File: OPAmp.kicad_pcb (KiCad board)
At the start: 2 copper layers, 100 x 100 mm, 20 parts, among them Q1 TIP120, Q2 TIP125, Q3 2N2219, Q4 2N2219

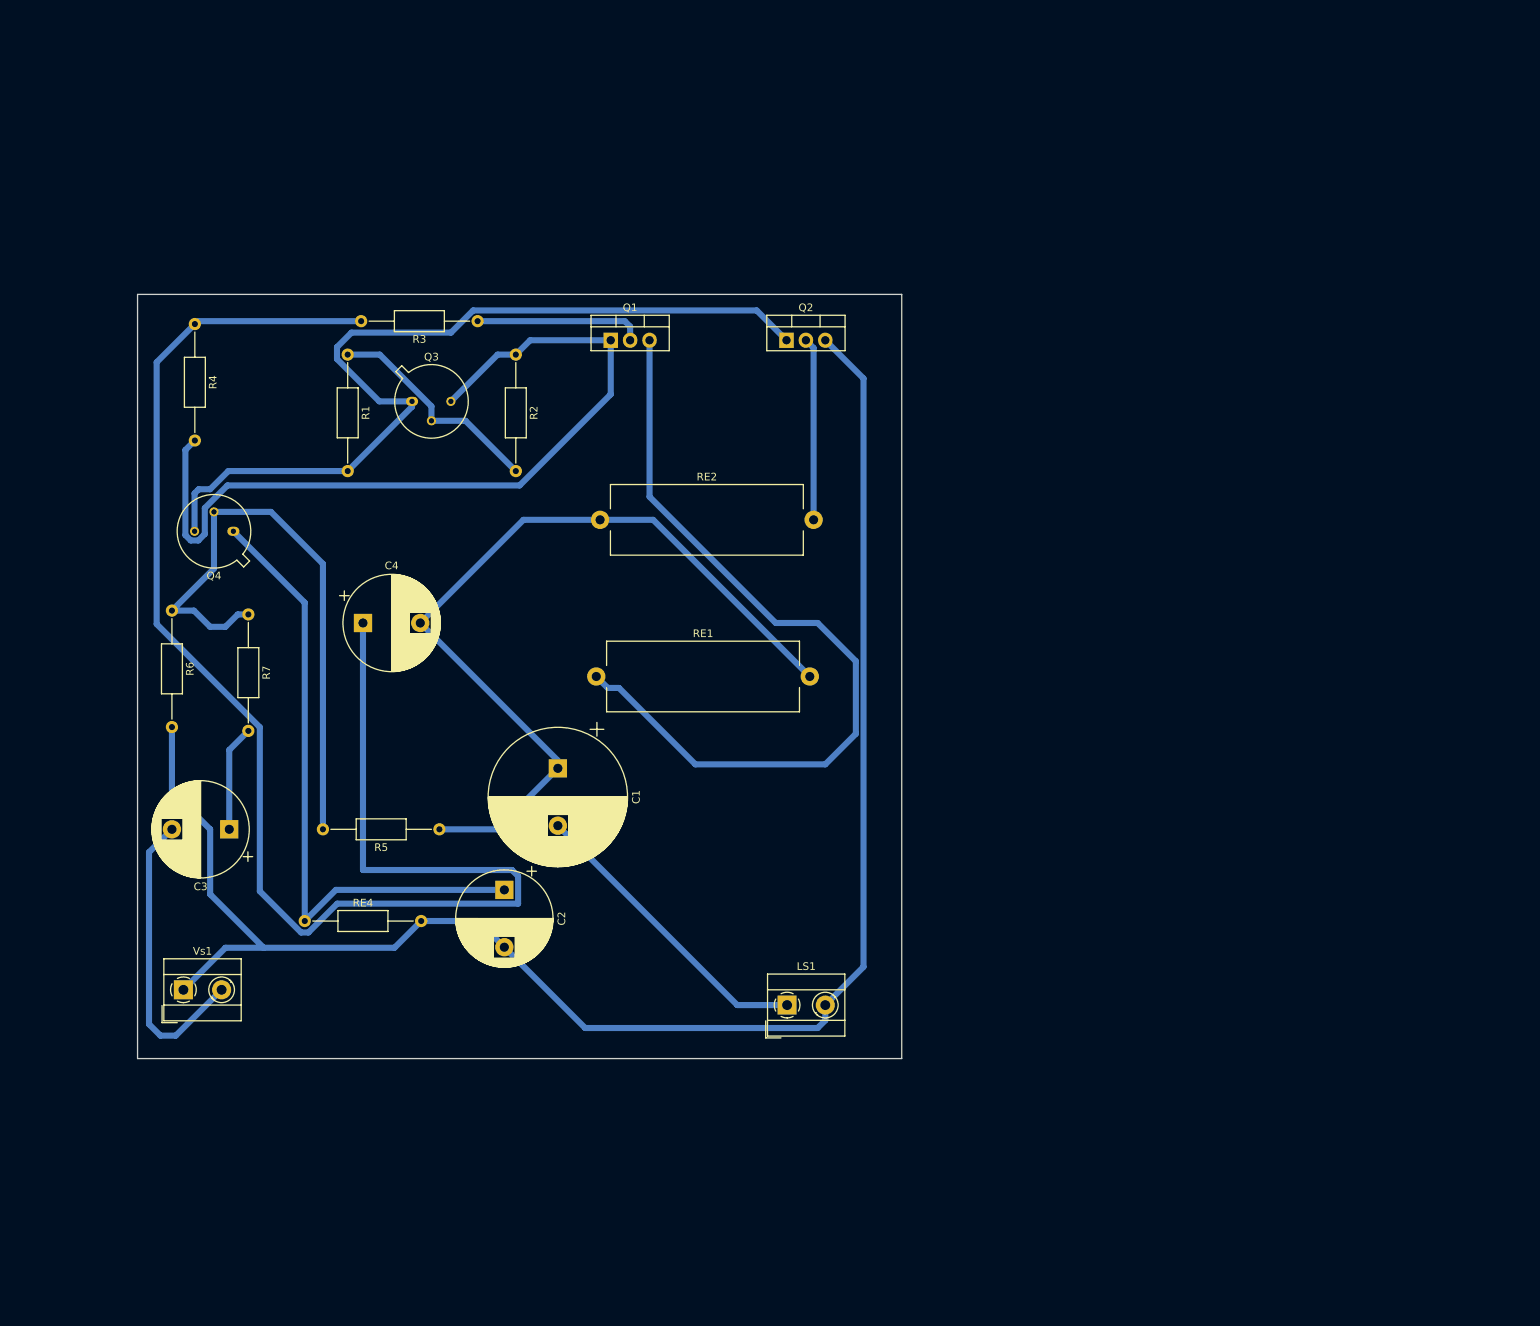
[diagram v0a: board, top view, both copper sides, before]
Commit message: Version 2
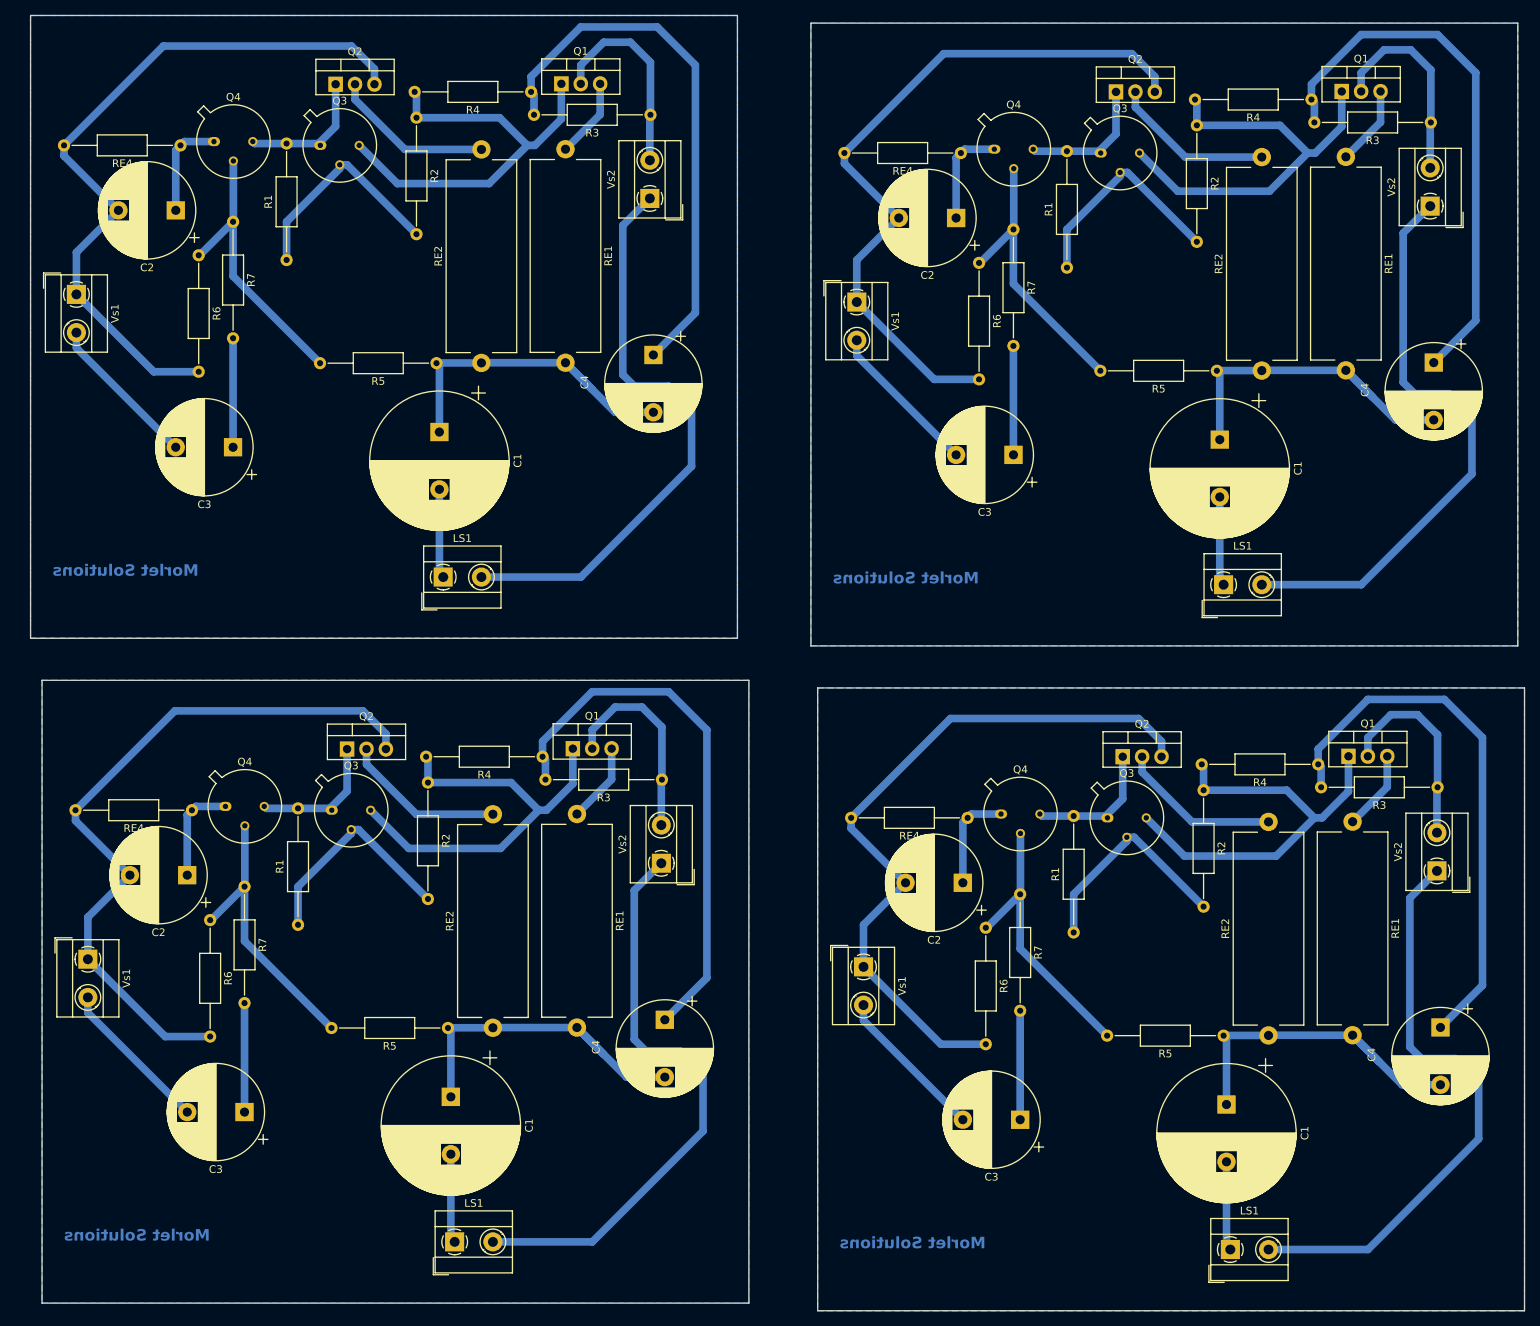
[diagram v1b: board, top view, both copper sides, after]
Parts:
- added C1: 4700uF, Capacitor_THT:CP_Radial_D18.0mm_P7.50mm, F.Cu at (142.0, 155.0)
- added C1: 4700uF, Capacitor_THT:CP_Radial_D18.0mm_P7.50mm, F.Cu at (140.5, 68.0)
- added C1: 4700uF, Capacitor_THT:CP_Radial_D18.0mm_P7.50mm, F.Cu at (243.5, 156.0)
- added C2: 100uF, Capacitor_THT:CP_Radial_D12.5mm_P7.50mm, F.Cu at (209.0, 127.0)
- added C2: 100uF, Capacitor_THT:CP_Radial_D12.5mm_P7.50mm, F.Cu at (106.0, 39.0)
- added C2: 100uF, Capacitor_THT:CP_Radial_D12.5mm_P7.50mm, F.Cu at (107.5, 126.0)
- added C3: 100uF, Capacitor_THT:CP_Radial_D12.5mm_P7.50mm, F.Cu at (115.0, 157.0)
- added C3: 100uF, Capacitor_THT:CP_Radial_D12.5mm_P7.50mm, F.Cu at (216.5, 158.0)
- added C3: 100uF, Capacitor_THT:CP_Radial_D12.5mm_P7.50mm, F.Cu at (113.5, 70.0)
- added C4: 100uF, Capacitor_THT:CP_Radial_D12.5mm_P7.50mm, F.Cu at (170.0, 144.9)
- added C4: 100uF, Capacitor_THT:CP_Radial_D12.5mm_P7.50mm, F.Cu at (168.5, 57.9)
- added C4: 100uF, Capacitor_THT:CP_Radial_D12.5mm_P7.50mm, F.Cu at (271.5, 145.9)
- added LS1: 8Ohm, TerminalBlock_MetzConnect:TerminalBlock_MetzConnect_Type055_RT01502HDWU_1x02_P5.00mm_Horizontal, F.Cu at (142.5, 174.0)
- added LS1: 8Ohm, TerminalBlock_MetzConnect:TerminalBlock_MetzConnect_Type055_RT01502HDWU_1x02_P5.00mm_Horizontal, F.Cu at (141.0, 87.0)
- added LS1: 8Ohm, TerminalBlock_MetzConnect:TerminalBlock_MetzConnect_Type055_RT01502HDWU_1x02_P5.00mm_Horizontal, F.Cu at (244.0, 175.0)
- added Q1: TIP120, Package_TO_SOT_THT:TO-220-3_Vertical, F.Cu at (156.5, 22.4)
- added Q1: TIP120, Package_TO_SOT_THT:TO-220-3_Vertical, F.Cu at (158.0, 109.4)
- added Q1: TIP120, Package_TO_SOT_THT:TO-220-3_Vertical, F.Cu at (259.5, 110.4)
- added Q2: TIP125, Package_TO_SOT_THT:TO-220-3_Vertical, F.Cu at (229.9, 110.5)
- added Q2: TIP125, Package_TO_SOT_THT:TO-220-3_Vertical, F.Cu at (128.4, 109.5)
- added Q2: TIP125, Package_TO_SOT_THT:TO-220-3_Vertical, F.Cu at (126.9, 22.5)
- added Q3: 2N2219, Package_TO_SOT_THT:TO-39-3, F.Cu at (124.9, 30.5)
- added Q3: 2N2219, Package_TO_SOT_THT:TO-39-3, F.Cu at (227.9, 118.5)
- added Q3: 2N2219, Package_TO_SOT_THT:TO-39-3, F.Cu at (126.4, 117.5)
- added Q4: 2N2219, Package_TO_SOT_THT:TO-39-3, F.Cu at (111.0, 30.0)
- added Q4: 2N2219, Package_TO_SOT_THT:TO-39-3, F.Cu at (112.5, 117.0)
- added Q4: 2N2219, Package_TO_SOT_THT:TO-39-3, F.Cu at (214.0, 118.0)
- added R1: 1kOhm, Resistor_THT:R_Axial_DIN0207_L6.3mm_D2.5mm_P15.24mm_Horizontal, F.Cu at (122.0, 132.5)
- added R1: 1kOhm, Resistor_THT:R_Axial_DIN0207_L6.3mm_D2.5mm_P15.24mm_Horizontal, F.Cu at (223.5, 133.5)
- added R1: 1kOhm, Resistor_THT:R_Axial_DIN0207_L6.3mm_D2.5mm_P15.24mm_Horizontal, F.Cu at (120.5, 45.5)
- added R2: 2.7kOhm, Resistor_THT:R_Axial_DIN0207_L6.3mm_D2.5mm_P15.24mm_Horizontal, F.Cu at (240.5, 114.9)
- added R2: 2.7kOhm, Resistor_THT:R_Axial_DIN0207_L6.3mm_D2.5mm_P15.24mm_Horizontal, F.Cu at (139.0, 113.9)
- added R2: 2.7kOhm, Resistor_THT:R_Axial_DIN0207_L6.3mm_D2.5mm_P15.24mm_Horizontal, F.Cu at (137.5, 26.9)
- added R3: 1.8kOhm, Resistor_THT:R_Axial_DIN0207_L6.3mm_D2.5mm_P15.24mm_Horizontal, F.Cu at (169.6, 113.5)
- added R3: 1.8kOhm, Resistor_THT:R_Axial_DIN0207_L6.3mm_D2.5mm_P15.24mm_Horizontal, F.Cu at (271.1, 114.5)
- added R3: 1.8kOhm, Resistor_THT:R_Axial_DIN0207_L6.3mm_D2.5mm_P15.24mm_Horizontal, F.Cu at (168.1, 26.5)
- added R4: 1.8kOhm, Resistor_THT:R_Axial_DIN0207_L6.3mm_D2.5mm_P15.24mm_Horizontal, F.Cu at (255.5, 111.5)
- added R4: 1.8kOhm, Resistor_THT:R_Axial_DIN0207_L6.3mm_D2.5mm_P15.24mm_Horizontal, F.Cu at (154.0, 110.5)
- added R4: 1.8kOhm, Resistor_THT:R_Axial_DIN0207_L6.3mm_D2.5mm_P15.24mm_Horizontal, F.Cu at (152.5, 23.5)
- added R5: 100kOhm, Resistor_THT:R_Axial_DIN0207_L6.3mm_D2.5mm_P15.24mm_Horizontal, F.Cu at (141.6, 146.0)
- added R5: 100kOhm, Resistor_THT:R_Axial_DIN0207_L6.3mm_D2.5mm_P15.24mm_Horizontal, F.Cu at (140.1, 59.0)
- added R5: 100kOhm, Resistor_THT:R_Axial_DIN0207_L6.3mm_D2.5mm_P15.24mm_Horizontal, F.Cu at (243.1, 147.0)
- added R6: 20kOhm, Resistor_THT:R_Axial_DIN0207_L6.3mm_D2.5mm_P15.24mm_Horizontal, F.Cu at (110.5, 131.9)
- added R6: 20kOhm, Resistor_THT:R_Axial_DIN0207_L6.3mm_D2.5mm_P15.24mm_Horizontal, F.Cu at (212.0, 132.9)
- added R6: 20kOhm, Resistor_THT:R_Axial_DIN0207_L6.3mm_D2.5mm_P15.24mm_Horizontal, F.Cu at (109.0, 44.9)
- added R7: 5.1kOhm, Resistor_THT:R_Axial_DIN0207_L6.3mm_D2.5mm_P15.24mm_Horizontal, F.Cu at (113.5, 40.5)
- added R7: 5.1kOhm, Resistor_THT:R_Axial_DIN0207_L6.3mm_D2.5mm_P15.24mm_Horizontal, F.Cu at (216.5, 128.5)
- added R7: 5.1kOhm, Resistor_THT:R_Axial_DIN0207_L6.3mm_D2.5mm_P15.24mm_Horizontal, F.Cu at (115.0, 127.5)
- added RE1: 1 Ohm, Resistor_THT:R_Axial_Power_L25.0mm_W9.0mm_P27.94mm, F.Cu at (157.0, 31.0)
- added RE1: 1 Ohm, Resistor_THT:R_Axial_Power_L25.0mm_W9.0mm_P27.94mm, F.Cu at (158.5, 118.0)
- added RE1: 1 Ohm, Resistor_THT:R_Axial_Power_L25.0mm_W9.0mm_P27.94mm, F.Cu at (260.0, 119.0)
- added RE2: 1 Ohm, Resistor_THT:R_Axial_Power_L25.0mm_W9.0mm_P27.94mm, F.Cu at (147.5, 146.0)
- added RE2: 1 Ohm, Resistor_THT:R_Axial_Power_L25.0mm_W9.0mm_P27.94mm, F.Cu at (146.0, 59.0)
- added RE2: 1 Ohm, Resistor_THT:R_Axial_Power_L25.0mm_W9.0mm_P27.94mm, F.Cu at (249.0, 147.0)
- added RE4: 470 Ohm, Resistor_THT:R_Axial_DIN0207_L6.3mm_D2.5mm_P15.24mm_Horizontal, F.Cu at (108.1, 117.5)
- added RE4: 470 Ohm, Resistor_THT:R_Axial_DIN0207_L6.3mm_D2.5mm_P15.24mm_Horizontal, F.Cu at (106.6, 30.5)
- added RE4: 470 Ohm, Resistor_THT:R_Axial_DIN0207_L6.3mm_D2.5mm_P15.24mm_Horizontal, F.Cu at (209.6, 118.5)
- added Vs1: Conn_01x02, TerminalBlock_MetzConnect:TerminalBlock_MetzConnect_Type055_RT01502HDWU_1x02_P5.00mm_Horizontal, F.Cu at (94.5, 137.0)
- added Vs1: Conn_01x02, TerminalBlock_MetzConnect:TerminalBlock_MetzConnect_Type055_RT01502HDWU_1x02_P5.00mm_Horizontal, F.Cu at (93.0, 50.0)
- added Vs1: Conn_01x02, TerminalBlock_MetzConnect:TerminalBlock_MetzConnect_Type055_RT01502HDWU_1x02_P5.00mm_Horizontal, F.Cu at (196.0, 138.0)
- added Vs2: Conn_01x02, TerminalBlock_MetzConnect:TerminalBlock_MetzConnect_Type055_RT01502HDWU_1x02_P5.00mm_Horizontal, F.Cu at (168.0, 37.4)
- added Vs2: Conn_01x02, TerminalBlock_MetzConnect:TerminalBlock_MetzConnect_Type055_RT01502HDWU_1x02_P5.00mm_Horizontal, F.Cu at (169.5, 124.4)
- added Vs2: Conn_01x02, TerminalBlock_MetzConnect:TerminalBlock_MetzConnect_Type055_RT01502HDWU_1x02_P5.00mm_Horizontal, F.Cu at (270.2, 38.4)
- added Vs2: Conn_01x02, TerminalBlock_MetzConnect:TerminalBlock_MetzConnect_Type055_RT01502HDWU_1x02_P5.00mm_Horizontal, F.Cu at (271.0, 125.4)
- moved R4 149.0 mm to (254.6, 24.5), turned to 180 degrees
- moved C4 144.2 mm to (270.6, 58.9), turned to -90 degrees
- moved RE4 132.2 mm to (208.7, 31.5), turned to 180 degrees
- moved R3 127.4 mm to (270.2, 27.5)
- moved Vs1 126.0 mm to (195.1, 51.0), turned to -90 degrees
- moved RE1 119.4 mm to (259.1, 32.0), turned to -90 degrees
- moved R5 118.1 mm to (242.2, 60.0)
- moved R6 115.0 mm to (211.1, 45.9)
- moved C3 113.7 mm to (215.6, 71.0)
- moved R7 112.1 mm to (215.6, 41.5)
- moved Q4 111.4 mm to (213.1, 31.0), turned to 0 degrees
- moved C2 106.0 mm to (208.1, 40.0), turned to 180 degrees
- moved Q1 101.0 mm to (258.6, 23.4)
- moved C1 96.7 mm to (242.6, 69.0)
- moved Q3 95.8 mm to (227.0, 31.5)
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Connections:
- net VCC renamed Net-(Q1-C)
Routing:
- net GND: track 220.9 -> 682.2 mm
- net Net-(Q1-B): track 110.1 -> 224.4 mm
- net Net-(C4-Pad1): track 198.0 -> 286.5 mm
- net Net-(Q3-B): track 29.4 -> 116.6 mm
- net Net-(Q1-C): track 22.0 -> 107.5 mm
- net Net-(Q4-B): track 78.6 -> 150.0 mm
- net Net-(C1-Pad1): track 110.3 -> 180.8 mm
- net Net-(Q1-E): track 106.3 -> 41.7 mm
- net Net-(Q2-C): track 23.9 -> 85.0 mm
- net Net-(Q2-B): track 114.9 -> 70.9 mm
- net Net-(C3-Pad1): track 13.9 -> 57.0 mm
- net Net-(Vs1-Pin_2): track 39.3 -> 81.5 mm
- net Net-(Q4-E): track 82.7 -> 53.4 mm
- net Net-(C1-Pad2): track 39.7 -> 46.7 mm
- added copper zone on B.Cu, net GND
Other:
- board size 100 x 100 mm -> 195.5 x 169.5 mm
- board text added: "Morlet Solutions"

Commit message: V3
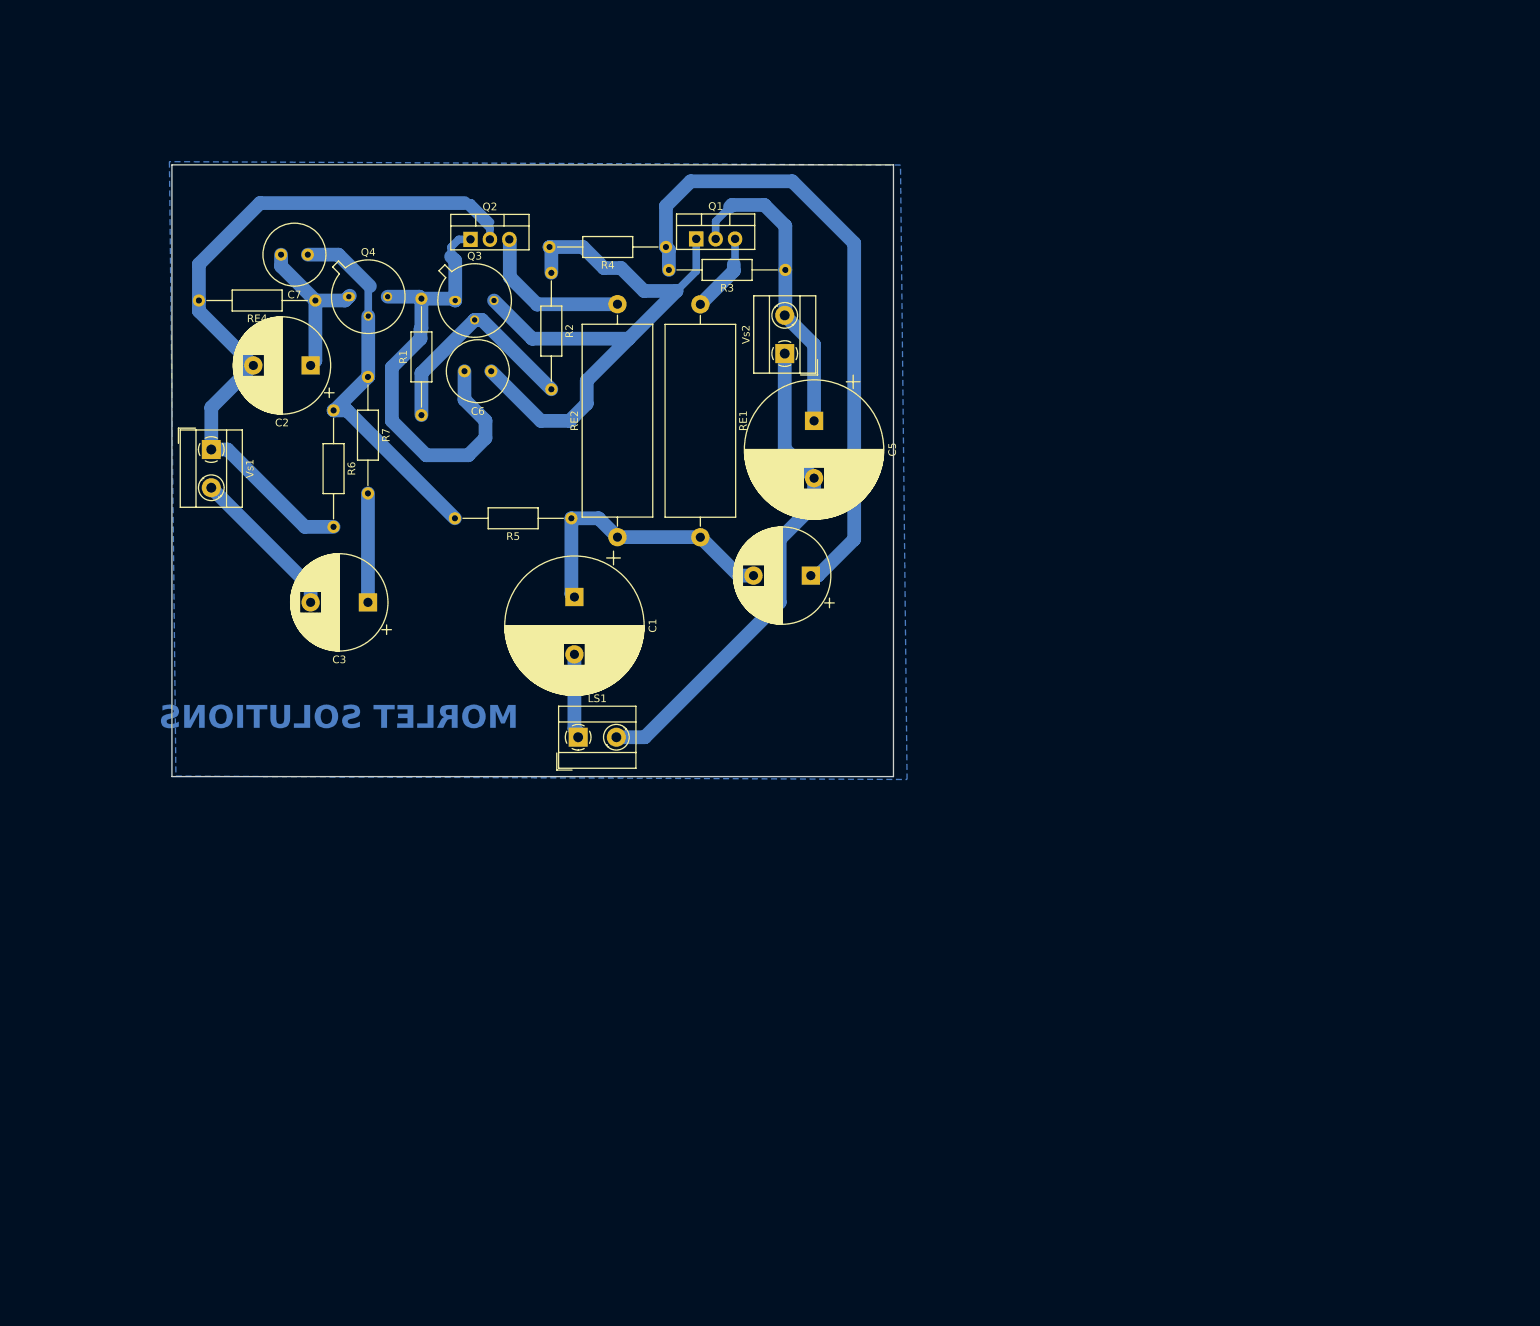
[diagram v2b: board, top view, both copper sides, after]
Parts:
- removed the C1 at (142.0, 155.0)
- removed the C1 at (140.5, 68.0)
- removed the C1 at (243.5, 156.0)
- removed the C2 at (209.0, 127.0)
- removed the C2 at (106.0, 39.0)
- removed the C2 at (107.5, 126.0)
- removed the C3 at (115.0, 157.0)
- removed the C3 at (216.5, 158.0)
- removed the C3 at (113.5, 70.0)
- removed the C4 at (170.0, 144.9)
- removed the C4 at (168.5, 57.9)
- removed the C4 at (271.5, 145.9)
- removed the LS1 at (142.5, 174.0)
- removed the LS1 at (141.0, 87.0)
- removed the LS1 at (244.0, 175.0)
- removed the Q1 at (156.5, 22.4)
- removed the Q1 at (158.0, 109.4)
- removed the Q1 at (259.5, 110.4)
- removed the Q2 at (229.9, 110.5)
- removed the Q2 at (128.4, 109.5)
- removed the Q2 at (126.9, 22.5)
- removed the Q3 at (124.9, 30.5)
- removed the Q3 at (227.9, 118.5)
- removed the Q3 at (126.4, 117.5)
- removed the Q4 at (111.0, 30.0)
- removed the Q4 at (112.5, 117.0)
- removed the Q4 at (214.0, 118.0)
- removed the R1 at (122.0, 132.5)
- removed the R1 at (223.5, 133.5)
- removed the R1 at (120.5, 45.5)
- removed the R2 at (240.5, 114.9)
- removed the R2 at (139.0, 113.9)
- removed the R2 at (137.5, 26.9)
- removed the R3 at (169.6, 113.5)
- removed the R3 at (271.1, 114.5)
- removed the R3 at (168.1, 26.5)
- removed the R4 at (255.5, 111.5)
- removed the R4 at (154.0, 110.5)
- removed the R4 at (152.5, 23.5)
- removed the R5 at (141.6, 146.0)
- removed the R5 at (140.1, 59.0)
- removed the R5 at (243.1, 147.0)
- removed the R6 at (110.5, 131.9)
- removed the R6 at (212.0, 132.9)
- removed the R6 at (109.0, 44.9)
- removed the R7 at (113.5, 40.5)
- removed the R7 at (216.5, 128.5)
- removed the R7 at (115.0, 127.5)
- removed the RE1 at (157.0, 31.0)
- removed the RE1 at (158.5, 118.0)
- removed the RE1 at (260.0, 119.0)
- removed the RE2 at (147.5, 146.0)
- removed the RE2 at (146.0, 59.0)
- removed the RE2 at (249.0, 147.0)
- removed the RE4 at (108.1, 117.5)
- removed the RE4 at (106.6, 30.5)
- removed the RE4 at (209.6, 118.5)
- removed the Vs1 at (94.5, 137.0)
- removed the Vs1 at (93.0, 50.0)
- removed the Vs1 at (196.0, 138.0)
- removed the Vs2 at (168.0, 37.4)
- removed the Vs2 at (169.5, 124.4)
- removed the Vs2 at (271.0, 125.4)
- added C5: 4700uF, Capacitor_THT:CP_Radial_D18.0mm_P7.50mm, F.Cu at (189.5, 66.5)
- added C6: 10pF, Capacitor_THT:C_Radial_D8.0mm_H7.0mm_P3.50mm, F.Cu at (147.3, 60.0)
- added C7: 10pF, Capacitor_THT:C_Radial_D8.0mm_H7.0mm_P3.50mm, F.Cu at (123.3, 44.8)
- C3: value 100uF -> 1uF
- RE1, RE2: footprint Resistor_THT:R_Axial_Power_L25.0mm_W9.0mm_P27.94mm -> Resistor_THT:R_Axial_Power_L25.0mm_W9.0mm_P30.48mm
- moved RE2 87.1 mm to (163.8, 81.8)
- moved C1 86.9 mm to (158.2, 89.6)
- moved LS1 86.8 mm to (158.7, 108.0)
- moved Vs2 86.6 mm to (185.7, 57.7)
- moved RE4 86.6 mm to (124.3, 50.8)
- moved C2 86.6 mm to (123.7, 59.3)
- moved C3 86.6 mm to (131.2, 90.3)
- moved Q2 86.6 mm to (144.6, 42.8)
- moved Q3 86.6 mm to (142.6, 50.8)
- moved Q4 86.6 mm to (128.7, 50.3)
- moved R1 86.6 mm to (138.2, 65.8)
- moved R2 86.6 mm to (155.2, 47.2)
- moved R3 86.6 mm to (185.8, 46.8)
- moved R4 86.6 mm to (170.2, 43.8)
- moved R5 86.6 mm to (157.8, 79.3)
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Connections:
- Q2 pad 2: Net-(Q2-C) -> GND
- Q2 pad 3: GND -> Net-(Q2-E)
- RE2 pad 2: Net-(Q2-C) -> Net-(Q2-E)
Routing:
- net GND: track 682.2 -> 163.0 mm
- net Net-(C4-Pad1): track 286.5 -> 84.2 mm
- net Net-(C1-Pad1): track 180.8 -> 37.4 mm
- net Net-(Q1-B): track 224.4 -> 85.8 mm
- net Net-(Q4-B): track 150.0 -> 50.0 mm
- net Net-(Q3-B): track 116.6 -> 29.1 mm
- net Net-(Q2-C): track 85.0 -> 0.00 mm
- net Net-(Q1-C): track 107.5 -> 40.6 mm
- net Net-(Vs1-Pin_2): track 81.5 -> 20.4 mm
- net Net-(C3-Pad1): track 57.0 -> 14.3 mm
- net Net-(C1-Pad2): track 46.7 -> 11.1 mm
- net Net-(Q4-E): track 53.4 -> 21.4 mm
- net Net-(Q1-E): track 41.7 -> 10.4 mm
- net Net-(Q2-E): track 0.00 -> 20.5 mm
- net Net-(Q2-B): track 70.9 -> 61.8 mm
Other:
- board size 195.5 x 169.5 mm -> 94.4 x 80 mm
- board text added: "MORLET SOLUTIONS"
- board text removed: "Morlet Solutions"
